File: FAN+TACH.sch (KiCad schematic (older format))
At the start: 8 parts, among them U3 VNLD5090

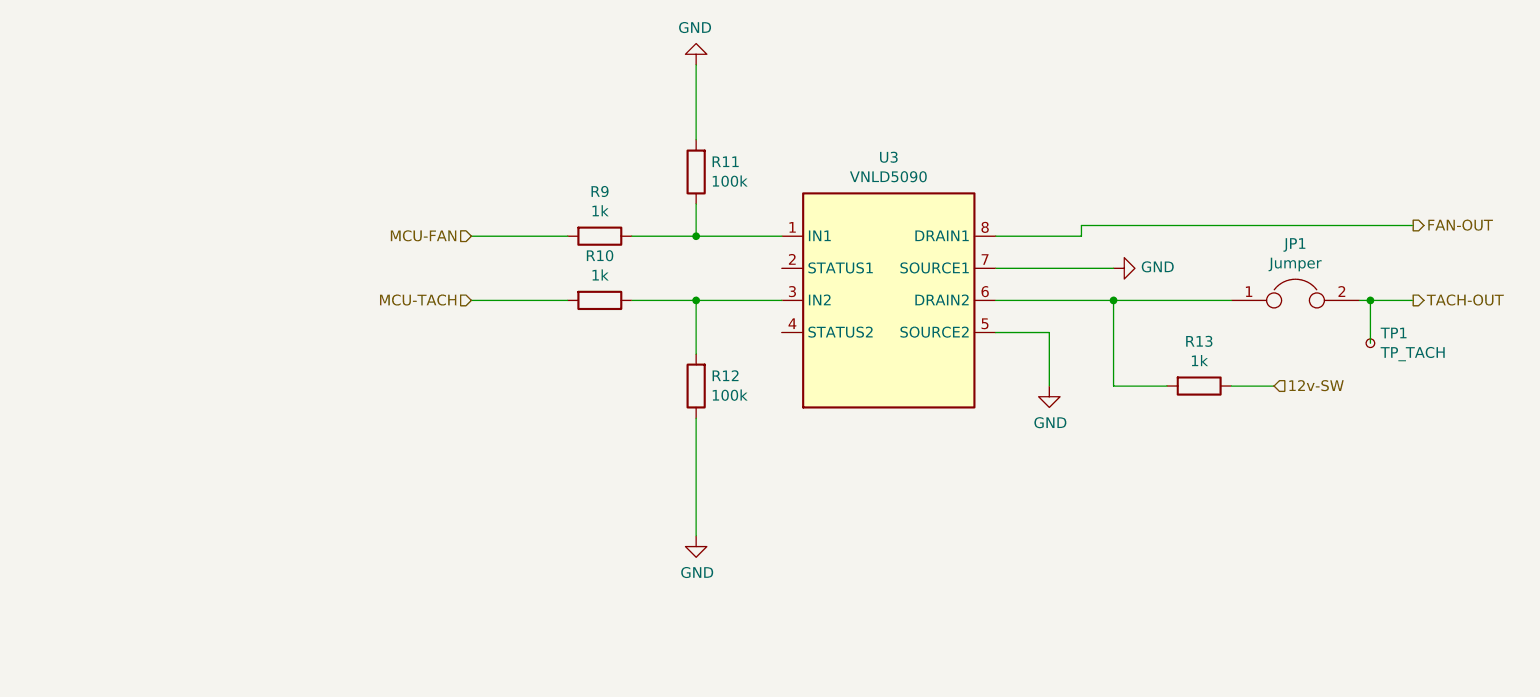
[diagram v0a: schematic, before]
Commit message: Update Schematic with a bunch of extra stuff
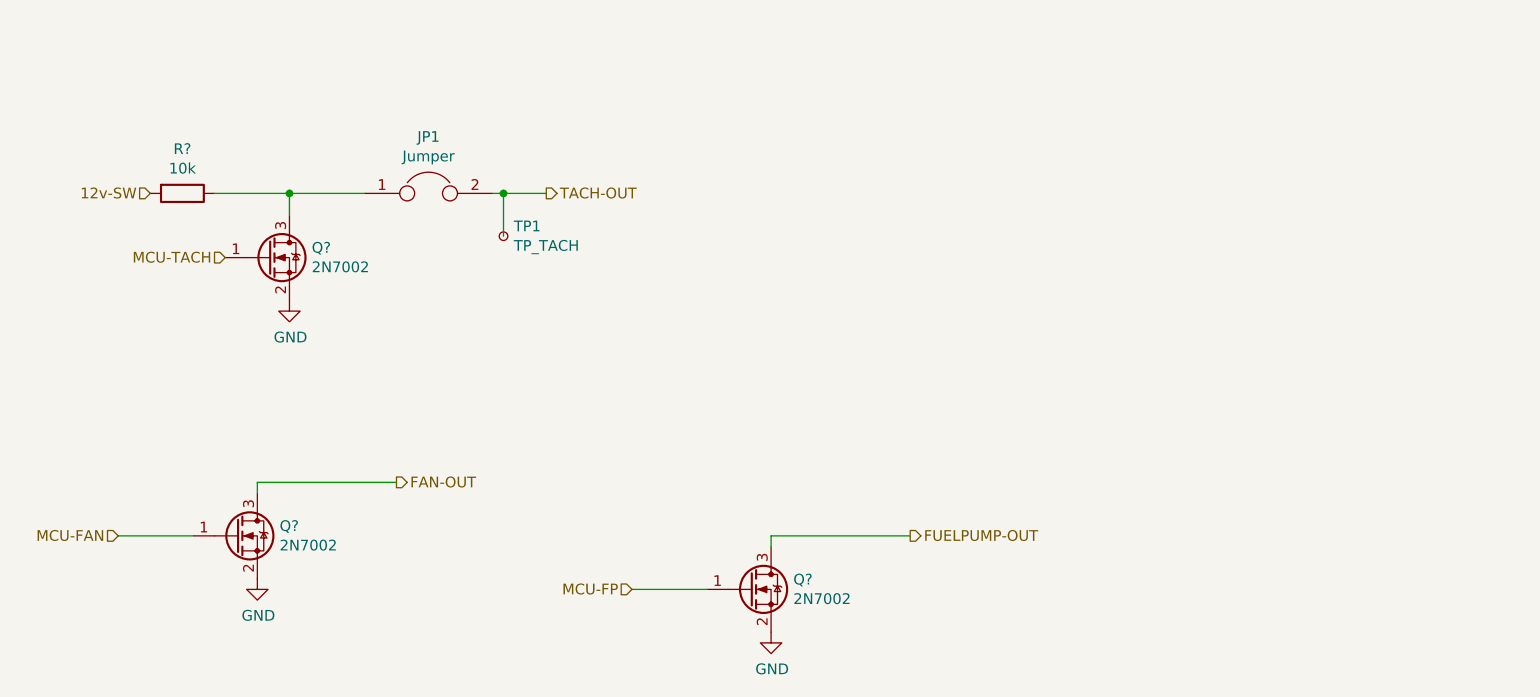
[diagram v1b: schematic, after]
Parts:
- removed R10, R13, R9: 1k, Resistor_SMD:R_0603_1608Metric_Pad0.98x0.95mm_HandSolder, symbol Device:R
- removed R11, R12: 100k, Resistor_SMD:R_0603_1608Metric_Pad0.98x0.95mm_HandSolder, symbol Device:R
- removed U3: VNLD5090, Package_SO:SOIC-8_3.9x4.9mm_P1.27mm, symbol speeduino_ic_automotive:VNLD5090
- added Q? (x3): 2N7002, Package_TO_SOT_SMD:SOT-23, symbol Transistor_FET:2N7002
- added R?: 10k, Resistor_SMD:R_0603_1608Metric_Pad0.98x0.95mm_HandSolder, symbol Device:R
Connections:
- net 12v-SW: now also R?.2
- net FAN-OUT: now also Q?.3 (D)
- net GND: now also Q?.2 (S), Q?.2 (S), Q?.2 (S)
- net MCU-FAN: now also Q?.1 (G)
- net MCU-TACH: now also Q?.1 (G)
- net at JP1.1: now also Q?.3 (D), R?.1
- new net FUELPUMP-OUT: Q?.3 (D)
- new net MCU-FP: Q?.1 (G)
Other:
- moved on the sheet: JP1, TP1
